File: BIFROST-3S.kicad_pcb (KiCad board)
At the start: 2 copper layers, 54 x 36 mm, 14 parts, among them J1 B6B-XH-A_LF__SN_, J2 560020-1020, J3 B4B-XH-A_LF__SN_, J4 XT30PW-M, J5 XT30PW-M

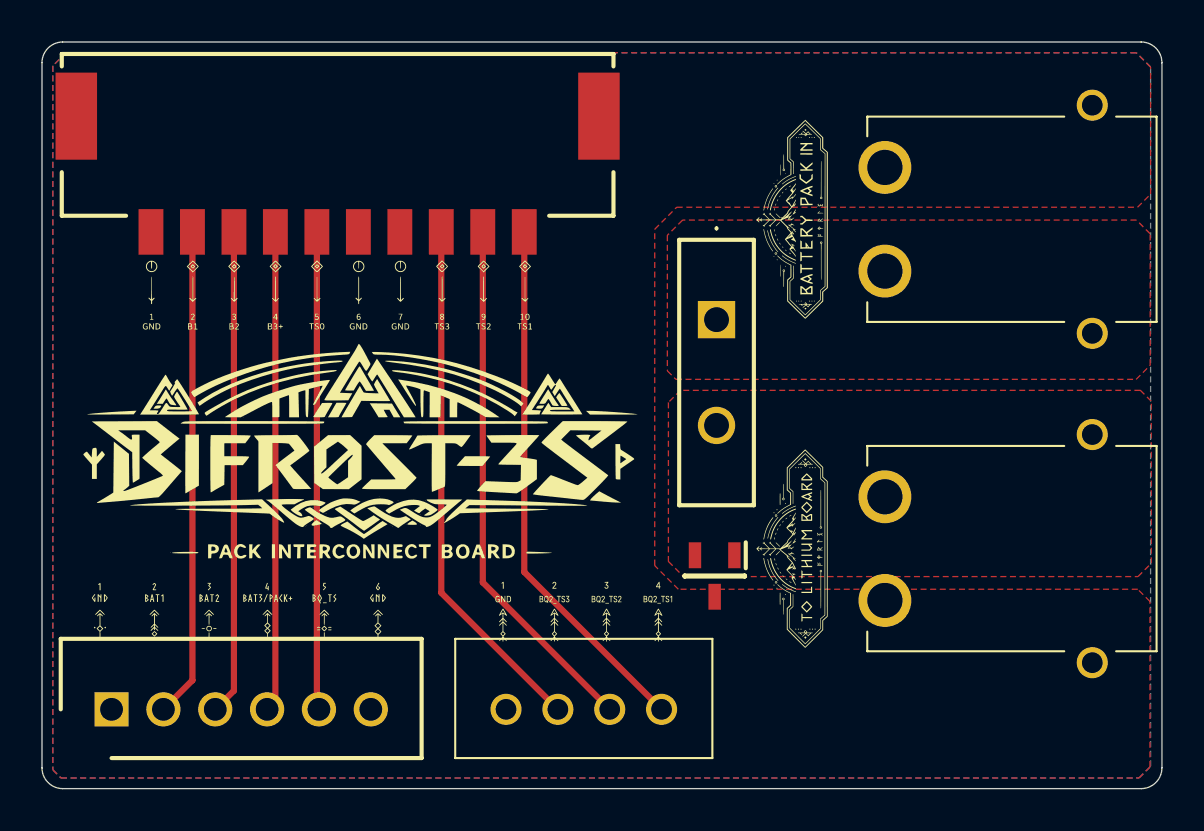
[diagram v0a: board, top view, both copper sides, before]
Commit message: Layout 3.1
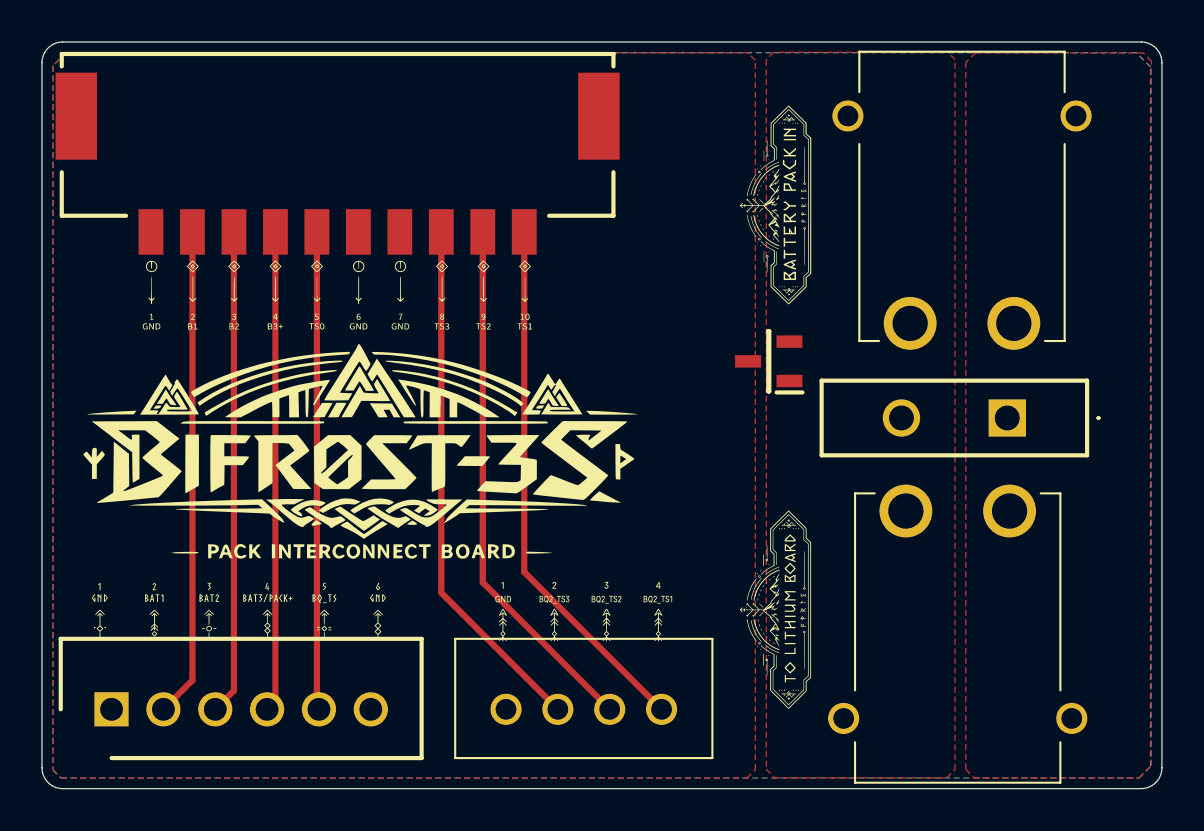
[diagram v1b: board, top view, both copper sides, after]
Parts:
- moved F1 14.8 mm to (161.2, 104.8), turned to 180 degrees
- moved D1 10.7 mm to (149.7, 102.1), turned to 180 degrees
- moved J4 4.75 mm to (158.8, 115.2), turned to 180 degrees
- moved G*** 3.05 mm to (150.1, 114.1)
- moved J5 2.37 mm to (159.0, 94.3), turned to 0 degrees
- moved G*** 1.06 mm to (150.4, 94.5)
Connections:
- J4 pad 1: /+BATT -> GND
- J4 pad 2: GND -> /+BATT
